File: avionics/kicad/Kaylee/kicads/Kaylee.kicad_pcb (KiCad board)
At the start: 4 copper layers, 90 x 65 mm, 67 parts

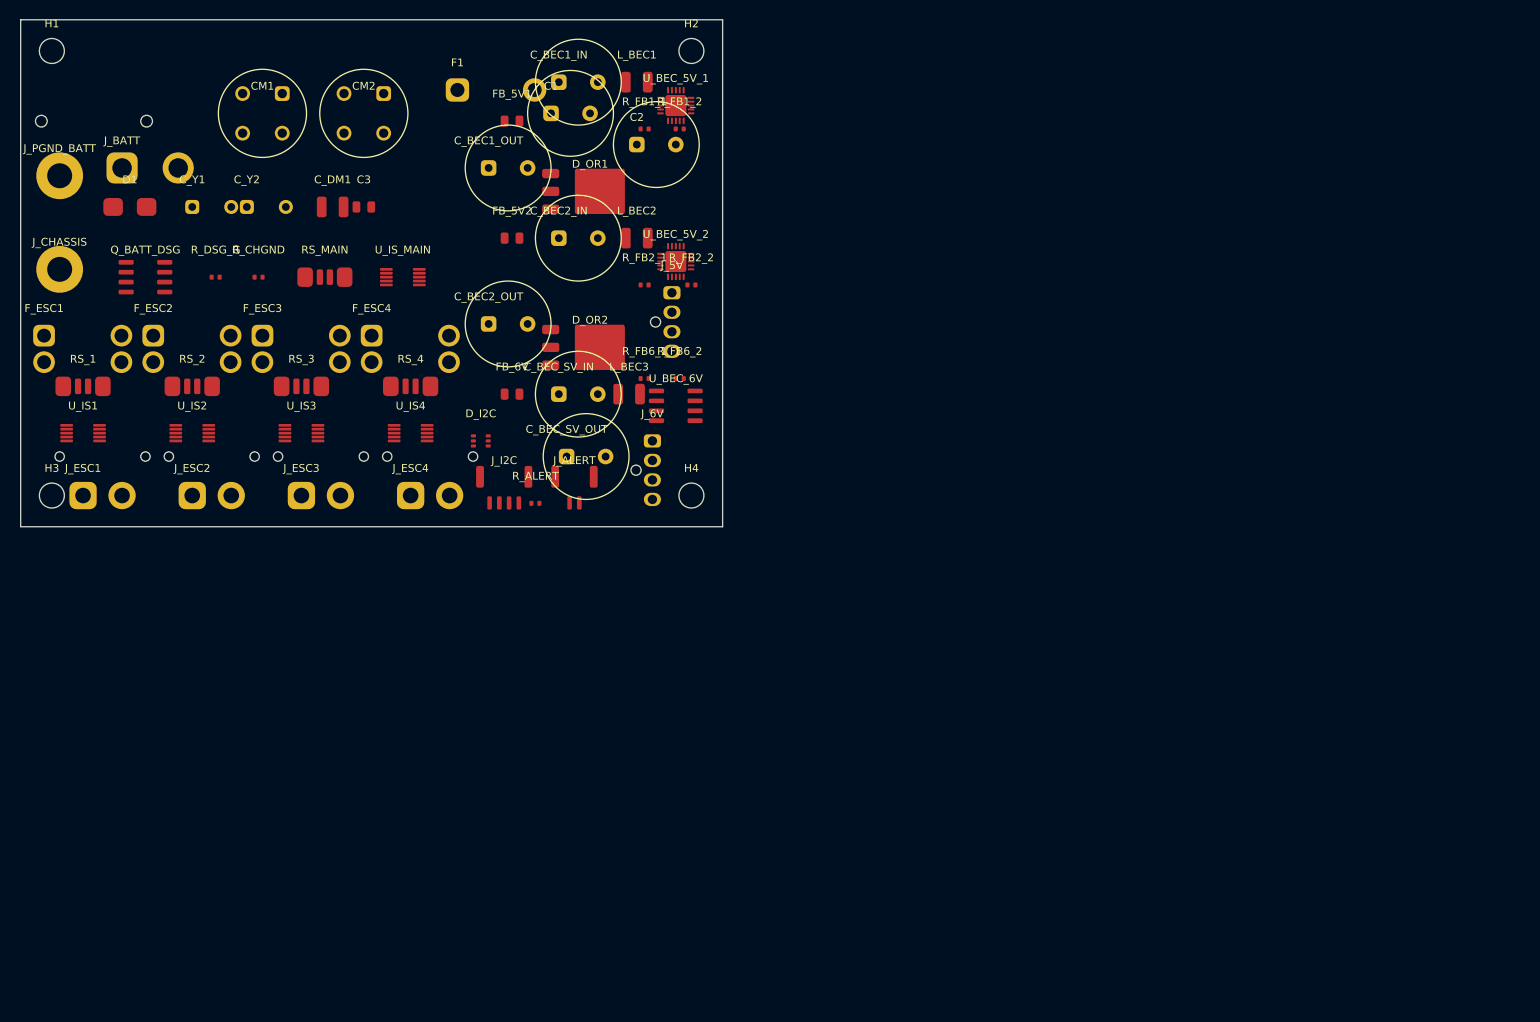
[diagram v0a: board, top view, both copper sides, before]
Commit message: lots of stuff
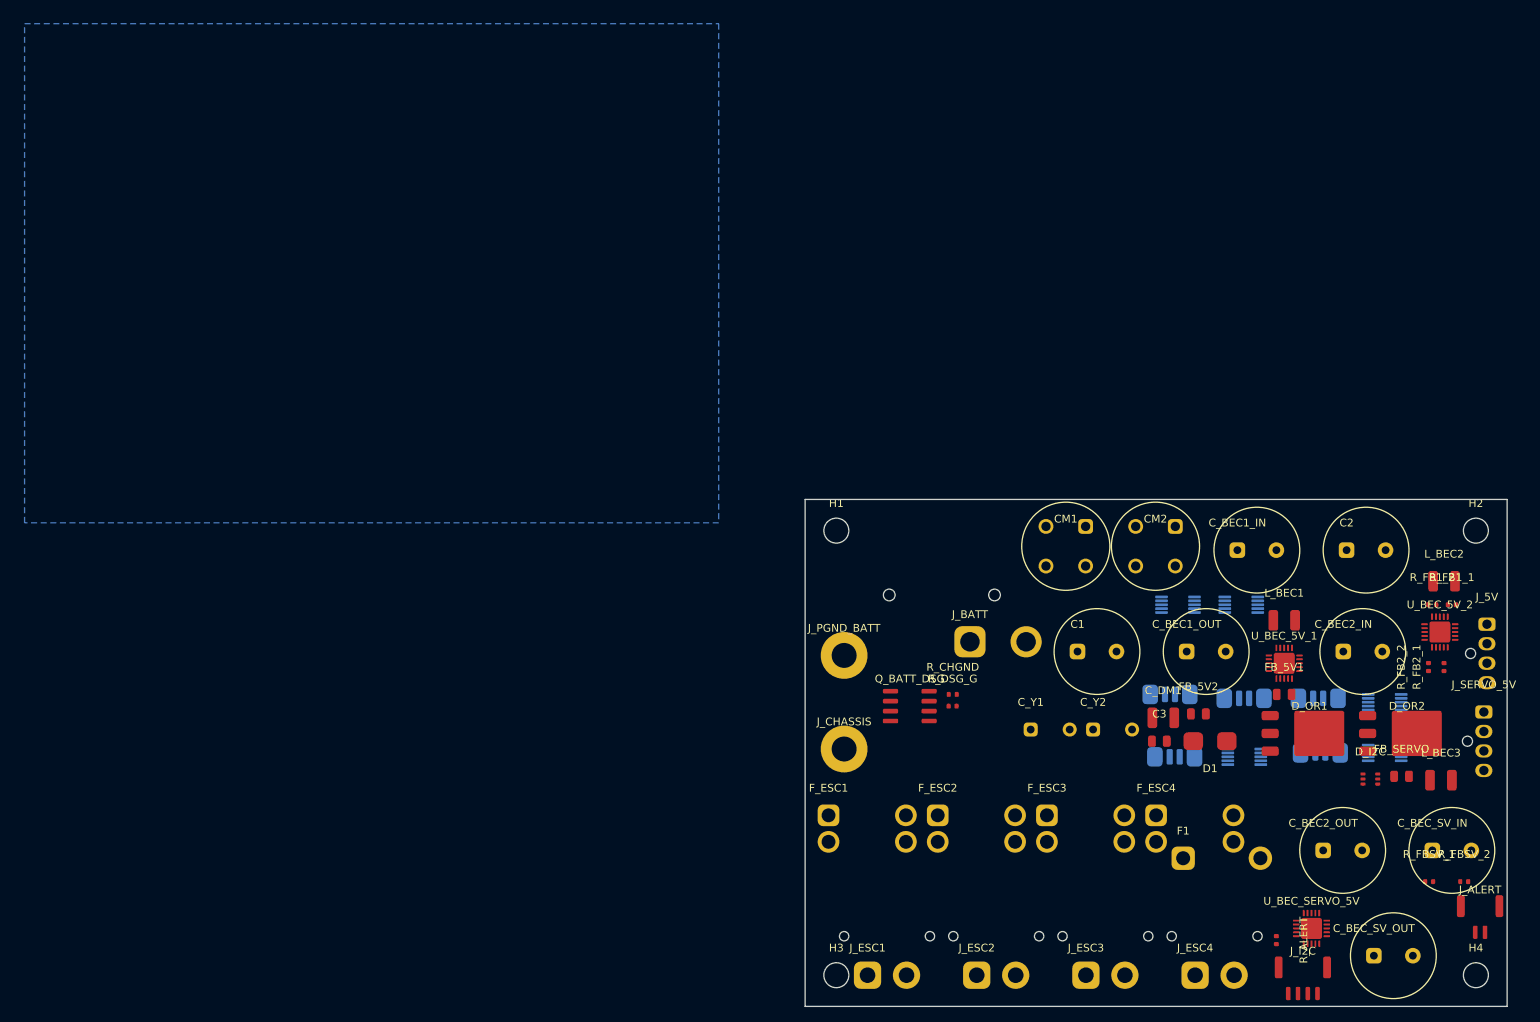
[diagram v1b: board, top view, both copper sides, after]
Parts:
- removed U_BEC_6V: TPS54540DDAR, Package_SO:SOIC-8_3.9x4.9mm_P1.27mm
- added U_BEC_SERVO_5V: TPS54620 sync buck 5.0V servo rail (pkg verify), Package_DFN_QFN:Texas_RGP0020D_VQFN-20-1EP_4x4mm_P0.5mm_EP2.7x2.7mm, F.Cu at (165.5, 116.5)
- RS_1, RS_2, RS_3, RS_4, RS_MAIN, U_IS1, U_IS2, U_IS3, U_IS4, U_IS_MAIN: moved to B.Cu
- moved U_IS1 171.9 mm to (174.9, 94.0), turned to 180 degrees
- moved RS_1 165.5 mm to (166.6, 94.0), turned to 180 degrees
- moved D1 154.5 mm to (152.5, 92.5), turned to 180 degrees
- moved RS_2 140.7 mm to (156.9, 87.0), turned to 180 degrees
- moved RS_MAIN 138.3 mm to (166.4, 87.0), turned to 180 degrees
- moved U_IS_MAIN 137.2 mm to (174.9, 87.5), turned to 180 degrees
- moved U_IS2 136.3 mm to (156.5, 75.0), turned to 180 degrees
- moved F1 135.5 mm to (149.1, 107.5)
- moved J_ALERT 128.5 mm to (187.1, 115.0)
- moved U_IS3 127.8 mm to (156.9, 94.5), turned to 180 degrees
- moved C_Y2 127.5 mm to (137.5, 91.0)
- moved C_Y1 126.7 mm to (129.5, 91.0)
- moved C_BEC2_OUT 126.5 mm to (167.0, 106.5)
- moved C_BEC_SV_IN 126.4 mm to (181.0, 106.5)
- moved C_DM1 125.0 mm to (146.5, 89.5)
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- renumbered FB_6V to FB_SERVO, J_6V to J_SERVO_5V, R_FB6_1 to R_FBSV_1, R_FB6_2 to R_FBSV_2
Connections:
- C_BEC_SV_IN pad 1: BEC6V_VIN_F -> BECSV_VIN_F
- C_BEC_SV_OUT pad 1: +6V -> 5V_SERVO
- FB_SERVO pad 2: BEC6V_VIN_F -> BECSV_VIN_F
- J_SERVO_5V pad 3: +6V -> 5V_SERVO
- J_SERVO_5V pad 4: +6V -> 5V_SERVO
- L_BEC1 pad 1: BEC1_VIN_F -> BEC1_PRE_OR
- L_BEC2 pad 1: BEC2_VIN_F -> BEC2_PRE_OR
- L_BEC3 pad 1: BEC6V_VIN_F -> 5V_SERVO
- L_BEC3 pad 2: BEC6V_SW -> BECSV_SW
- R_FB1_1 pad 2: (no net) -> BEC1_FB
- R_FB1_2 pad 1: (no net) -> BEC1_FB
- R_FB2_1 pad 2: (no net) -> BEC2_FB
- R_FB2_2 pad 1: (no net) -> BEC2_FB
- R_FBSV_1 pad 1: +6V -> 5V_SERVO
- R_FBSV_1 pad 2: (no net) -> BECSV_FB
- R_FBSV_2 pad 1: (no net) -> BECSV_FB
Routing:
- added copper zone on B.Cu, net VBAT
- removed copper zone on In2.Cu, net VBAT
